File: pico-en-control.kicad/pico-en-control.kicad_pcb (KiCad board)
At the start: 2 copper layers, 17 parts, among them J1 JST-PH2 Bat, J2 Pico Pin 1-7, J3 Pico Pin 40-34, SW1 SW_Push, U1 SN74HC74N, U2 PCF8563T, Y1 Crystal

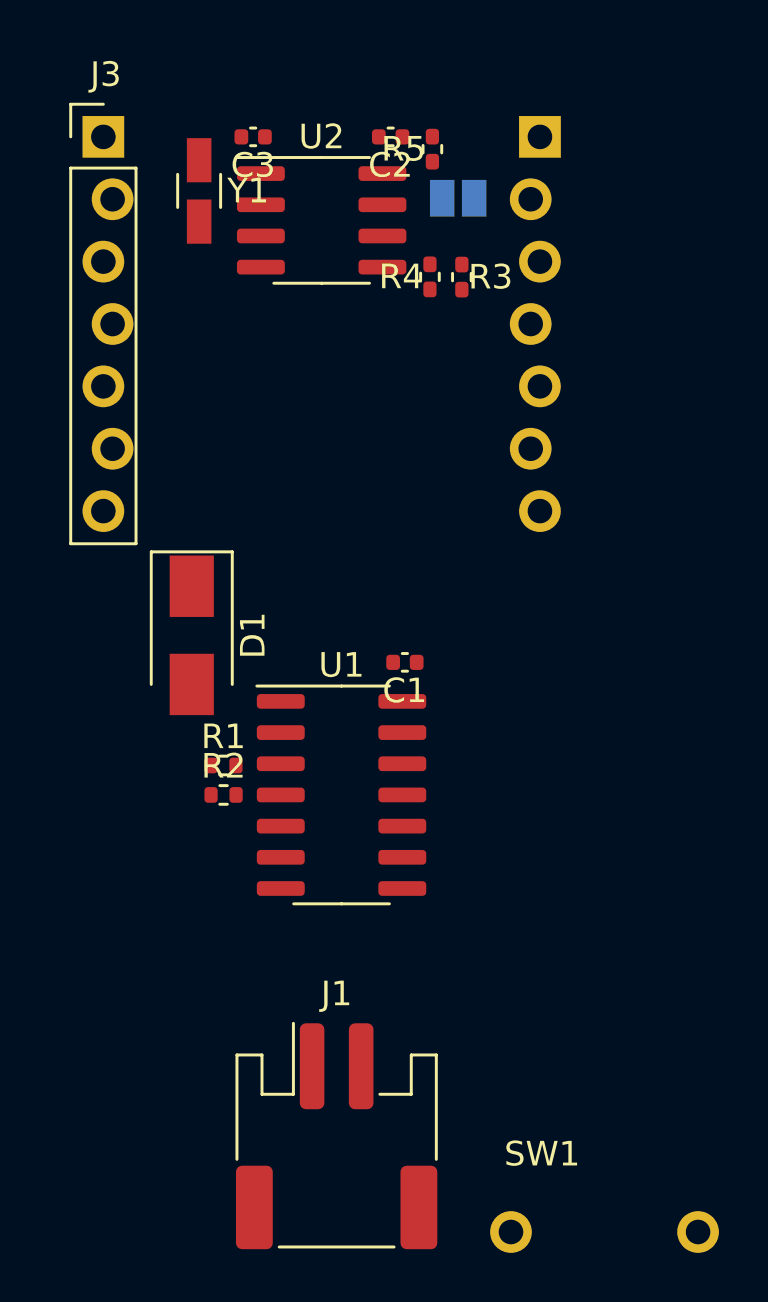
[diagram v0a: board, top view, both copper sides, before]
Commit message: draft routing
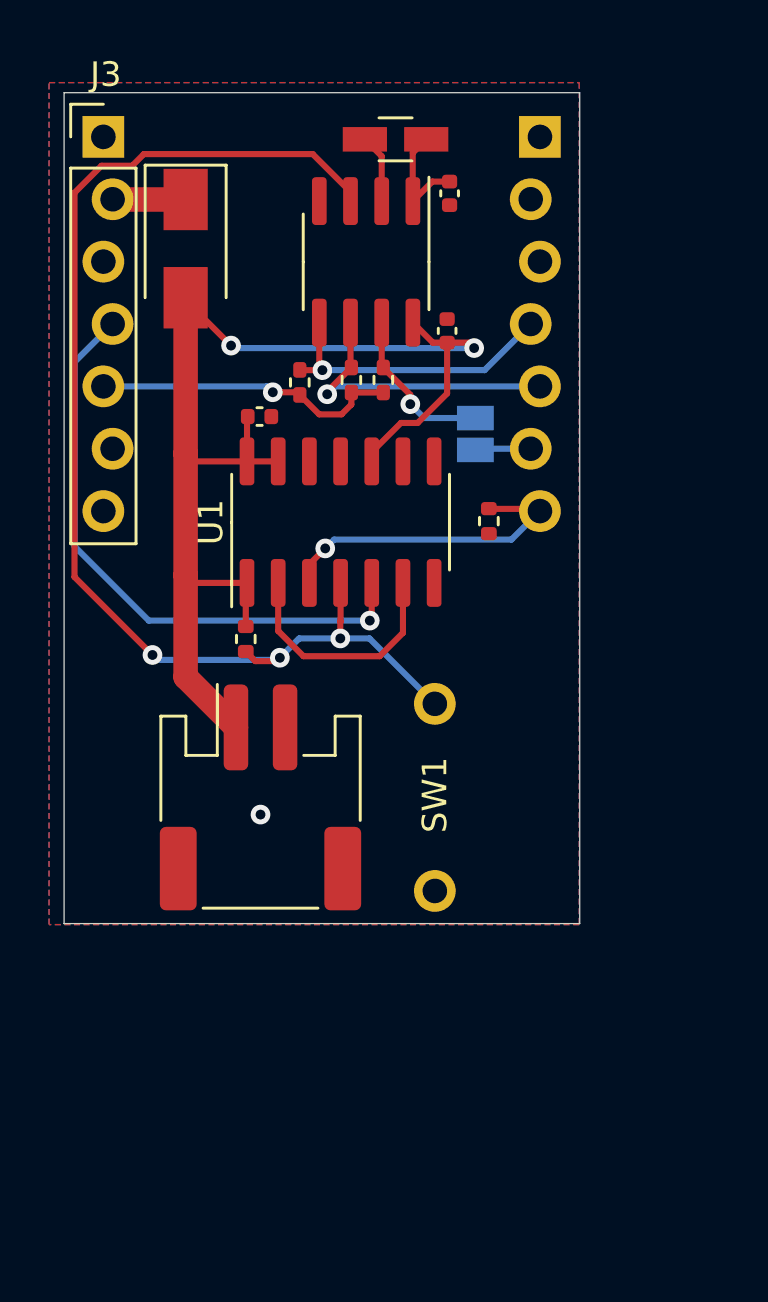
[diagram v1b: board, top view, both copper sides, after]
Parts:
- moved D1 15.8 mm to (103.3, 104.5)
- moved R1 14.7 mm to (115.7, 115.7), turned to 90 degrees
- moved SW1 14.2 mm to (113.5, 130.7), turned to 90 degrees
- moved J1 14.1 mm to (106.4, 126.9)
- moved C1 11.6 mm to (106.4, 111.4), turned to 0 degrees
- moved U1 11.1 mm to (109.7, 115.7), turned to 90 degrees
- moved JP1 9.63 mm to (115.2, 112.1), turned to 90 degrees
- moved R5 9.61 mm to (111.4, 109.9), turned to -90 degrees
- moved C3 8.32 mm to (114.1, 102.3), turned to 90 degrees
- moved Y1 8.27 mm to (111.9, 100.1), turned to 180 degrees
- moved C2 8.23 mm to (114.0, 107.9), turned to 90 degrees
- moved R4 6.82 mm to (108.0, 110.0), turned to -90 degrees
- moved R2 6.41 mm to (105.8, 120.5), turned to -90 degrees
- moved R3 6.15 mm to (110.1, 109.9)
- moved U2 2.48 mm to (110.7, 105.1), turned to -90 degrees
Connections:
- J2 pad 2: /GP2 -> unconnected-(J2-Pad2)
- J2 pad 6: /GP4_DONE -> /GP4_CLKOUT
- J2 pad 7: unconnected-(J2-Pad7) -> /GP5_DONE
- JP1 pad 1: /GP2 -> /GP4_CLKOUT
- R1 pad 2: /GP4_DONE -> /GP5_DONE
- R5 pad 1: +BATT -> /CLKOUT
- R5 pad 2: /CLKOUT -> +3V3
- U1 pad 3: /GP4_DONE -> /GP5_DONE
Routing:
- net +BATT: track 0.00 -> 50.6 mm, vias 0 -> 2
- net /1~{PRE}: track 0.00 -> 50.0 mm, vias 0 -> 3
- net /3V3_EN: track 0.00 -> 24.5 mm, vias 0 -> 1
- net /GP5_DONE: track 0.00 -> 13.2 mm, vias 0 -> 1
- net +3V3: track 0.00 -> 12.4 mm, vias 0 -> 1
- net /SDA: track 0.00 -> 12.2 mm, vias 0 -> 1
- net /SCL: track 0.00 -> 12.1 mm, vias 0 -> 1
- net Net-(U1-Pad2): track 0.00 -> 9.89 mm
- net /CLKOUT: track 0.00 -> 6.74 mm, vias 0 -> 1
- net Net-(C3-Pad2): track 0.00 -> 4.57 mm
- net /VSYS: track 0.00 -> 2.98 mm
- net Net-(U2-Pad2): track 0.00 -> 2.80 mm
- net /GP4_CLKOUT: track 0.00 -> 2.27 mm
- net GND: vias 0 -> 1
- added copper zone on B.Cu, net GND
- added copper zone on F.Cu, net GND
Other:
- board outline added: 21 x 33.8 mm
